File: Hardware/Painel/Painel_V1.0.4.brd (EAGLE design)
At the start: 44.4 x 25.9 mm, 18 parts, among them J1 J5MM, Q1 AO3401, Q2 AO3401, Q3 AO3401

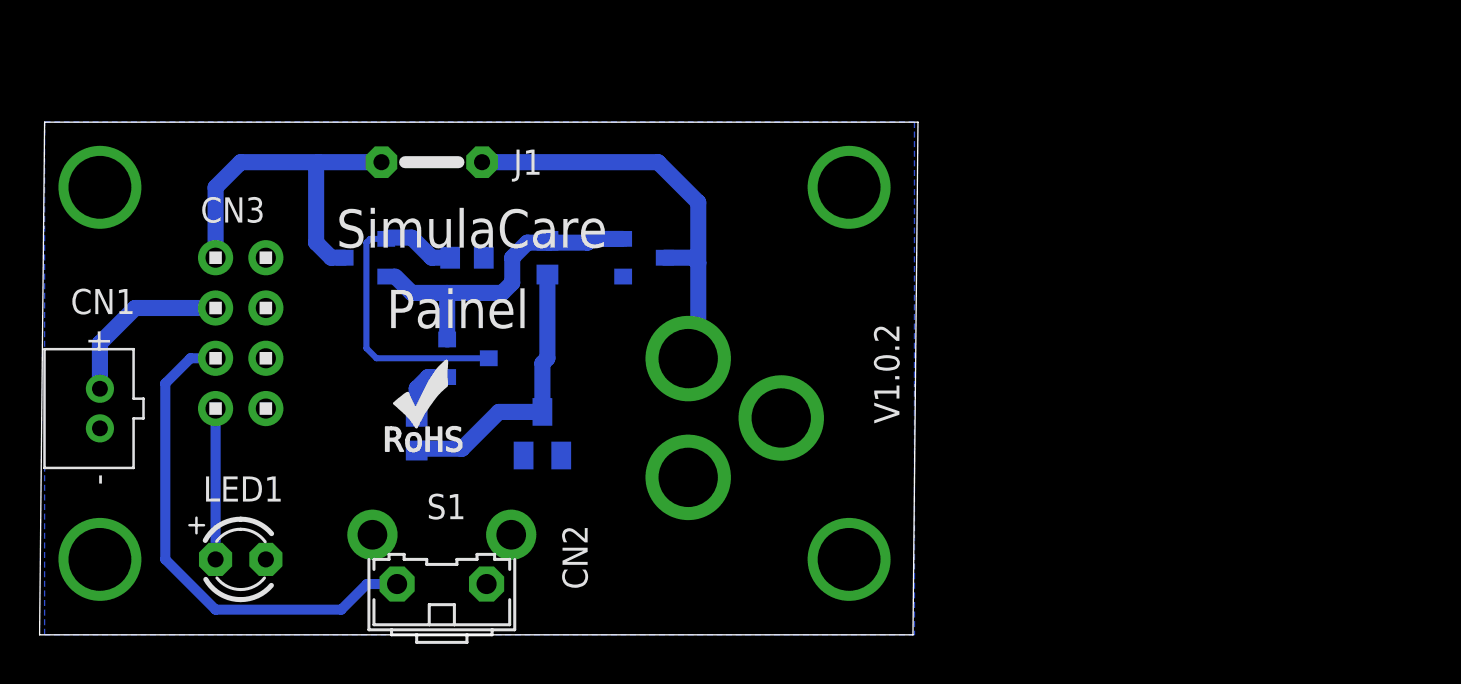
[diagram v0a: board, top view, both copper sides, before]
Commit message: V1.0.2
PCB v1.0.2
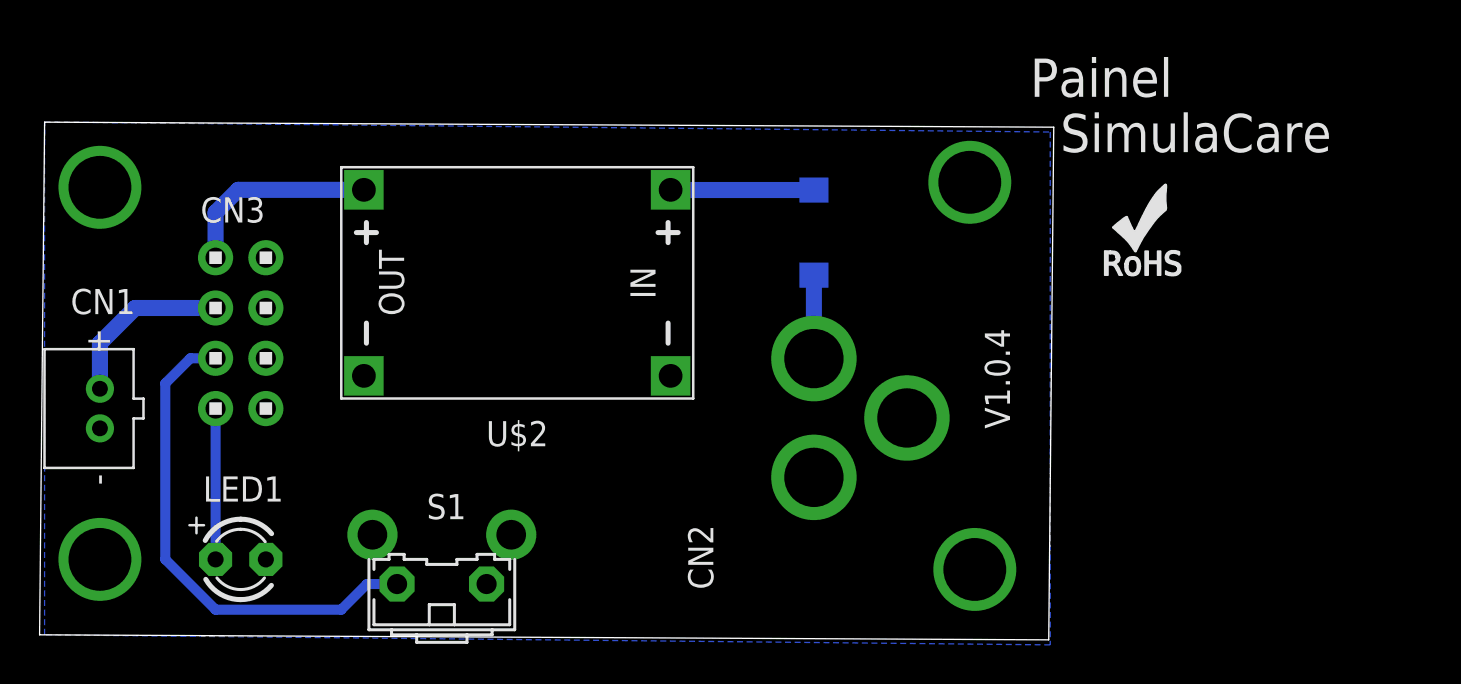
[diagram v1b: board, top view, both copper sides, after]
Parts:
- removed D3: (no value), diode:SOT23
- removed J1: J5MM, jumper:05
- removed Q1, Q2, Q3: AO3401, SparkFun-DiscreteSemi:SOT23-3
- removed R1, R2, R3: (no value), resistor:R0603
- added D1: 1A/40V/500mV, SparkFun-DiscreteSemi:SMA-DIODE
- added U$2: DC-DC-STEP-DOWN-MP2307, diy-modules:DC-DC-STEP-DOWN-MP2307
- moved U$1 37.4 mm to (52.3, 18.0)
- moved H4 6.37 mm to (46.0, 3.30)
- moved CN2 6.35 mm to (37.8, 0.25)
- moved H3 6.10 mm to (45.7, 22.9)
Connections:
- removed net N$3: Q2.1, R2.1
- removed net N$4: Q2.3, Q3.1, R3.1
- removed net VCC: CN2.PWR, J1.1, Q1.3
- net GND: now also U$2.IN-, U$2.OUT-; no longer D3.1, Q1.1, R3.2
- net N$1: now also CN2.PWR, D1.A; no longer Q1.2, Q2.2, Q3.2, R1.2
- net N$2: now also D1.C, U$2.IN+; no longer D3.3, R1.1, R2.2
- net VOUT: now also U$2.OUT+; no longer J1.2, Q3.3
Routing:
- net VCC: track 21.7 -> 0.00 mm
- net N$4: track 16.5 -> 0.00 mm
- net N$1: track 16.7 -> 4.22 mm
- net VOUT: track 18.3 -> 10.3 mm
- net N$2: track 14.5 -> 7.24 mm
- net N$3: track 3.21 -> 0.00 mm
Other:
- board size 44.4 x 25.9 mm -> 51.2 x 26.2 mm
- board text added: "V1.0.4"
- board text removed: "V1.0.2"
